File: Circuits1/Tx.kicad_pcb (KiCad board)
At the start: 2 copper layers, 43.2 x 51.4 mm, 54 parts, among them CON1 USB-MINI-B, P1 CONN_3X2, SW1 SW_PUSH, SW2 Power Select, U1 ATMEGA32U4, U2 LD1117, U3 NRF24L01+, U4 MPU-6050, X1 QUARTZ, X2 QUARTZ

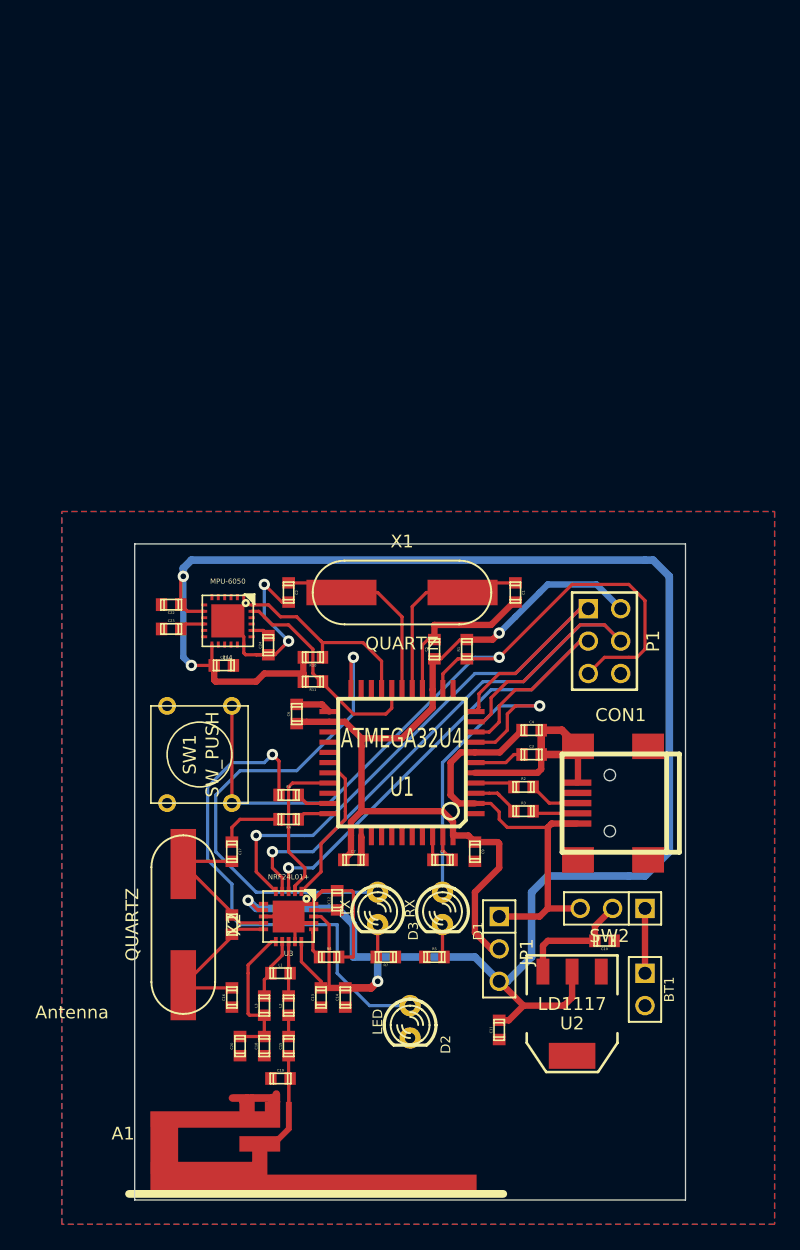
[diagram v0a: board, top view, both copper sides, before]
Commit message: Neatened Schematics and Final PCB
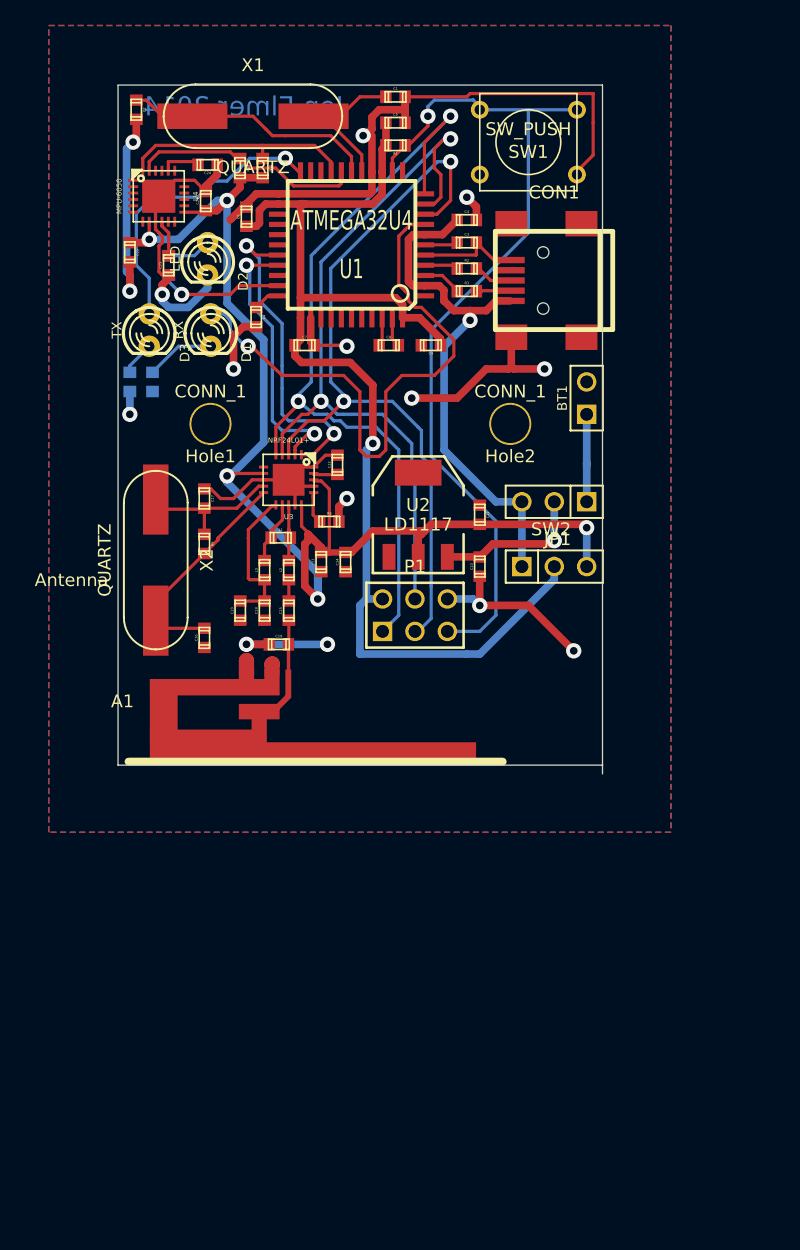
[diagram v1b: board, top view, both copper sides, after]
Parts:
- added Hole1: CONN_1, Drill3mm, F.Cu at (151.4, 51.6)
- added Hole2: CONN_1, Drill3mm, F.Cu at (174.9, 51.6)
- R5, R6, R7: moved to B.Cu
- moved D2 61.9 mm to (151.1, 38.6)
- moved SW1 54.5 mm to (176.3, 29.5), turned to 180 degrees
- moved R5 50.2 mm to (146.8, 48.3), turned to 90 degrees
- moved R7 49.3 mm to (145.0, 48.3), turned to 90 degrees
- moved D1 48.8 mm to (151.4, 44.2)
- moved D3 48.7 mm to (146.6, 44.2)
- moved BT1 46.6 mm to (180.8, 49.5), turned to 90 degrees
- moved R6 42.6 mm to (148.1, 39.1), turned to 270 degrees
- moved C5 41.4 mm to (165.9, 27.9), turned to 0 degrees
- moved CON1 41.3 mm to (178.3, 40.3)
- moved R3 41.0 mm to (171.4, 41.1)
- moved U2 40.9 mm to (167.6, 58.7), turned to 0 degrees
- moved R2 40.9 mm to (171.4, 39.4)
- moved U1 40.8 mm to (162.4, 37.5)
- moved R11 40.7 mm to (153.7, 31.5), turned to 270 degrees
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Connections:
- U4 pad 9: (no net) -> GND
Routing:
- net GND: track 100.3 -> 168.6 mm, vias 2 -> 15
- net 3V3: track 161.2 -> 112.7 mm, vias 4 -> 5
- net N-000002: track 39.6 -> 3.47 mm, vias 1 -> 0
- net VCC: track 72.2 -> 93.4 mm
- net N-0000012: track 26.6 -> 46.6 mm
- net N-000009: track 38.9 -> 23.4 mm
- net /ICSP Header/SCK: track 45.3 -> 59.7 mm, vias 1 -> 2
- net /Radio/CE: track 11.7 -> 25.3 mm, vias 0 -> 2
- net /ICSP Header/MISO: track 51.3 -> 63.3 mm, vias 1 -> 2
- net /Radio/CSN: track 12.3 -> 21.9 mm, vias 0 -> 2
- net N-000001: track 2.70 -> 10.1 mm, vias 0 -> 1
- net N-000008: track 16.8 -> 23.6 mm
- net N-0000052: track 12.1 -> 18.3 mm
- net RESET: track 62.9 -> 68.4 mm
- net /ICSP Header/MOSI: track 54.5 -> 58.7 mm, vias 1 -> 2
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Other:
- board size 43.2 x 51.4 mm -> 38 x 54 mm
- net class Ant: via_dia 0.889 -> 1.2; via_drill 0.635 -> 0.8
- net class Default: via_dia 0.889 -> 1.2; via_drill 0.635 -> 0.8
- net class FAT added: clearance 0.254, trace_width 1.2, via_dia 1.2, via_drill 0.8
- net class Power: via_dia 0.889 -> 1.2; via_drill 0.635 -> 0.8
- net class Power (thin): via_dia 0.889 -> 1.2; via_drill 0.635 -> 0.8
- board text added: "Jon Elmer 2014"
